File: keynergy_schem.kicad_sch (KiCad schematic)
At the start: 39 parts, among them J1 Conn_01x03_Pin, J2 Conn_01x03_Pin, J3 Conn_01x04_Pin, J4 Conn_01x03_Pin, J5 Conn_01x02_Pin, J6 Conn_01x03_Pin, J7 Conn_01x02_Pin, J8 Conn_01x03_Pin

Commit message: new
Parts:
- removed D1, D10, D11, D2, D3, D4, D5, D6, D7, D8, D9: D, Diode_THT:D_DO-35_SOD27_P7.62mm_Horizontal, symbol Device:D
- removed J2, J4, J6, J8: Conn_01x03_Pin, Connector_PinHeader_2.54mm:PinHeader_1x03_P2.54mm_Vertical, symbol Connector:Conn_01x03_Pin
- removed J5, J7: Conn_01x02_Pin, Connector_PinHeader_2.54mm:PinHeader_1x02_P2.54mm_Vertical, symbol Connector:Conn_01x02_Pin
- added C2: C_Polarized_Small, Capacitor_THT:CP_Radial_D8.0mm_P3.50mm, symbol Device:C_Polarized_Small
- added D1, D2, D3, D4: 1N5818, Diode_THT:D_DO-41_SOD81_P10.16mm_Horizontal, symbol Diode:1N5818
- added K12, K13, K14, K15, K16, K17, K18, K19, K20: ~, project library:Solenoid Key, symbol Key_symbol:Solenoid_Key
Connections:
- net Col 5-2 is gone; now on net Column 1: K9.4 (Bin)
- net Row 5-1 is gone; now on net Column 2: K10.4 (Bin)
- net Row 5-2 is gone; now on net Column 3: K11.4 (Bin)
- net Coil 2-1: now also K8.2 (C2); no longer K7.2 (C2)
- net Coil 5-1: now also K19.2 (C2); no longer K9.2 (C2)
- net Coil 5-2: now also K17.1 (C1); no longer K8.1 (C1)
- net Col 1-1: no longer K1.4 (Bin)
- net Col 1-2: no longer K2.4 (Bin)
- net Col 1-3: no longer K3.4 (Bin)
- net Col 1-4: no longer K4.4 (Bin)
- net Row 1: now also K1.3 (Bout), K2.3 (Bout), K3.3 (Bout), K4.3 (Bout)
- net Row 2: now also K5.3 (Bout), K6.3 (Bout), K7.3 (Bout), K8.3 (Bout)
- net Row 5: now also K17.3 (Bout), K18.3 (Bout), K19.3 (Bout), K20.3 (Bout)
- net Row 3: now reaches K11.3 (Bout)
- net Row 3: now also K10.3 (Bout), K9.3 (Bout), K12.3 (Bout)
- net Coil 3-2: now reaches K9.1 (C1)
- net Coil 3-2: no longer K8.2 (C2)
- net Coil 5-3 renamed Coil 3-1
- net Coil 5-4: no longer names the net of K10.1 (C1)
- net Coil 5-4: now also K9.2 (C2)
- net Col 2-1 renamed Column 1
- net Column 1: now also K1.4 (Bin), K13.4 (Bin), K17.4 (Bin)
- net Col 2-2 renamed Column 2
- net Column 2: now also K2.4 (Bin), K14.4 (Bin), K18.4 (Bin)
- net Col 2-3 renamed Column 3
- net Column 3: now also K3.4 (Bin), K15.4 (Bin), K19.4 (Bin)
- net Col 5-1 renamed Column 4
- net Column 4: now also K4.4 (Bin), K12.4 (Bin), K16.4 (Bin), K20.4 (Bin)
- new net: K17.2 (C2), K18.1 (C1)
- new net: K7.2 (C2), K8.1 (C1)
- new net: C2.2, D3.1 (K), D4.2 (A)
- new net: D1.2 (A), D3.2 (A)
- new net: K13.2 (C2), K14.1 (C1)
- new net: K14.2 (C2), K15.1 (C1)
- new net: C2.1, D2.1 (K), D4.1 (K)
- new net: D1.1 (K), D2.2 (A)
- new net: K18.2 (C2), K19.1 (C1)
- new net Coil 4-1: K15.2 (C2)
- new net Coil 4-2: K13.1 (C1)
- new net Row 4: K13.3 (Bout), K14.3 (Bout), K15.3 (Bout), K16.3 (Bout)
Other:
- note removed: "Row 1, Col 1-4"
- note removed: "Row 2-4, Col 1-3"
- note removed: "Row 2/3 - 4/5, Col 5"
- note removed: "Row 5, Col 1/2-3"
- moved on the sheet: A2, BT1, C1, D12, D13, D14, D15, J1, J3, K10, K11, K5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

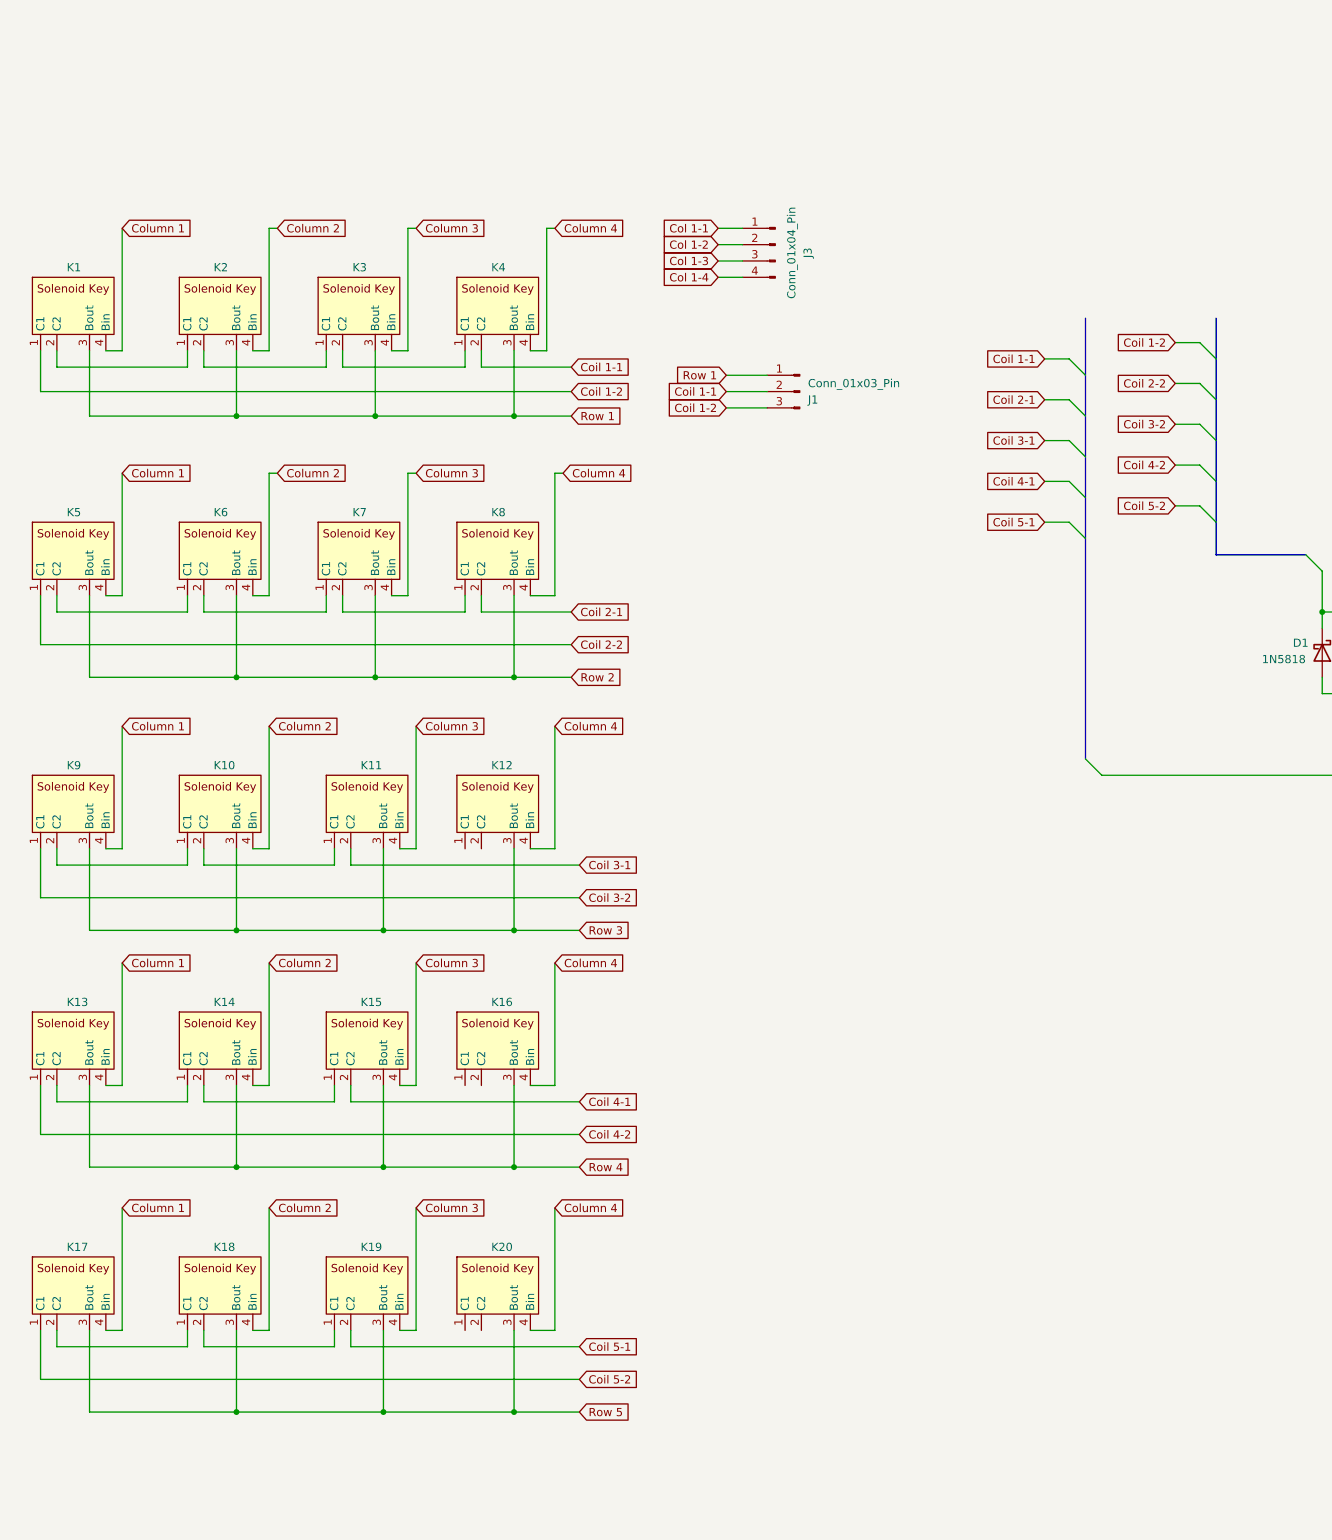
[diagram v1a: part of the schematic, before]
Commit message: new update
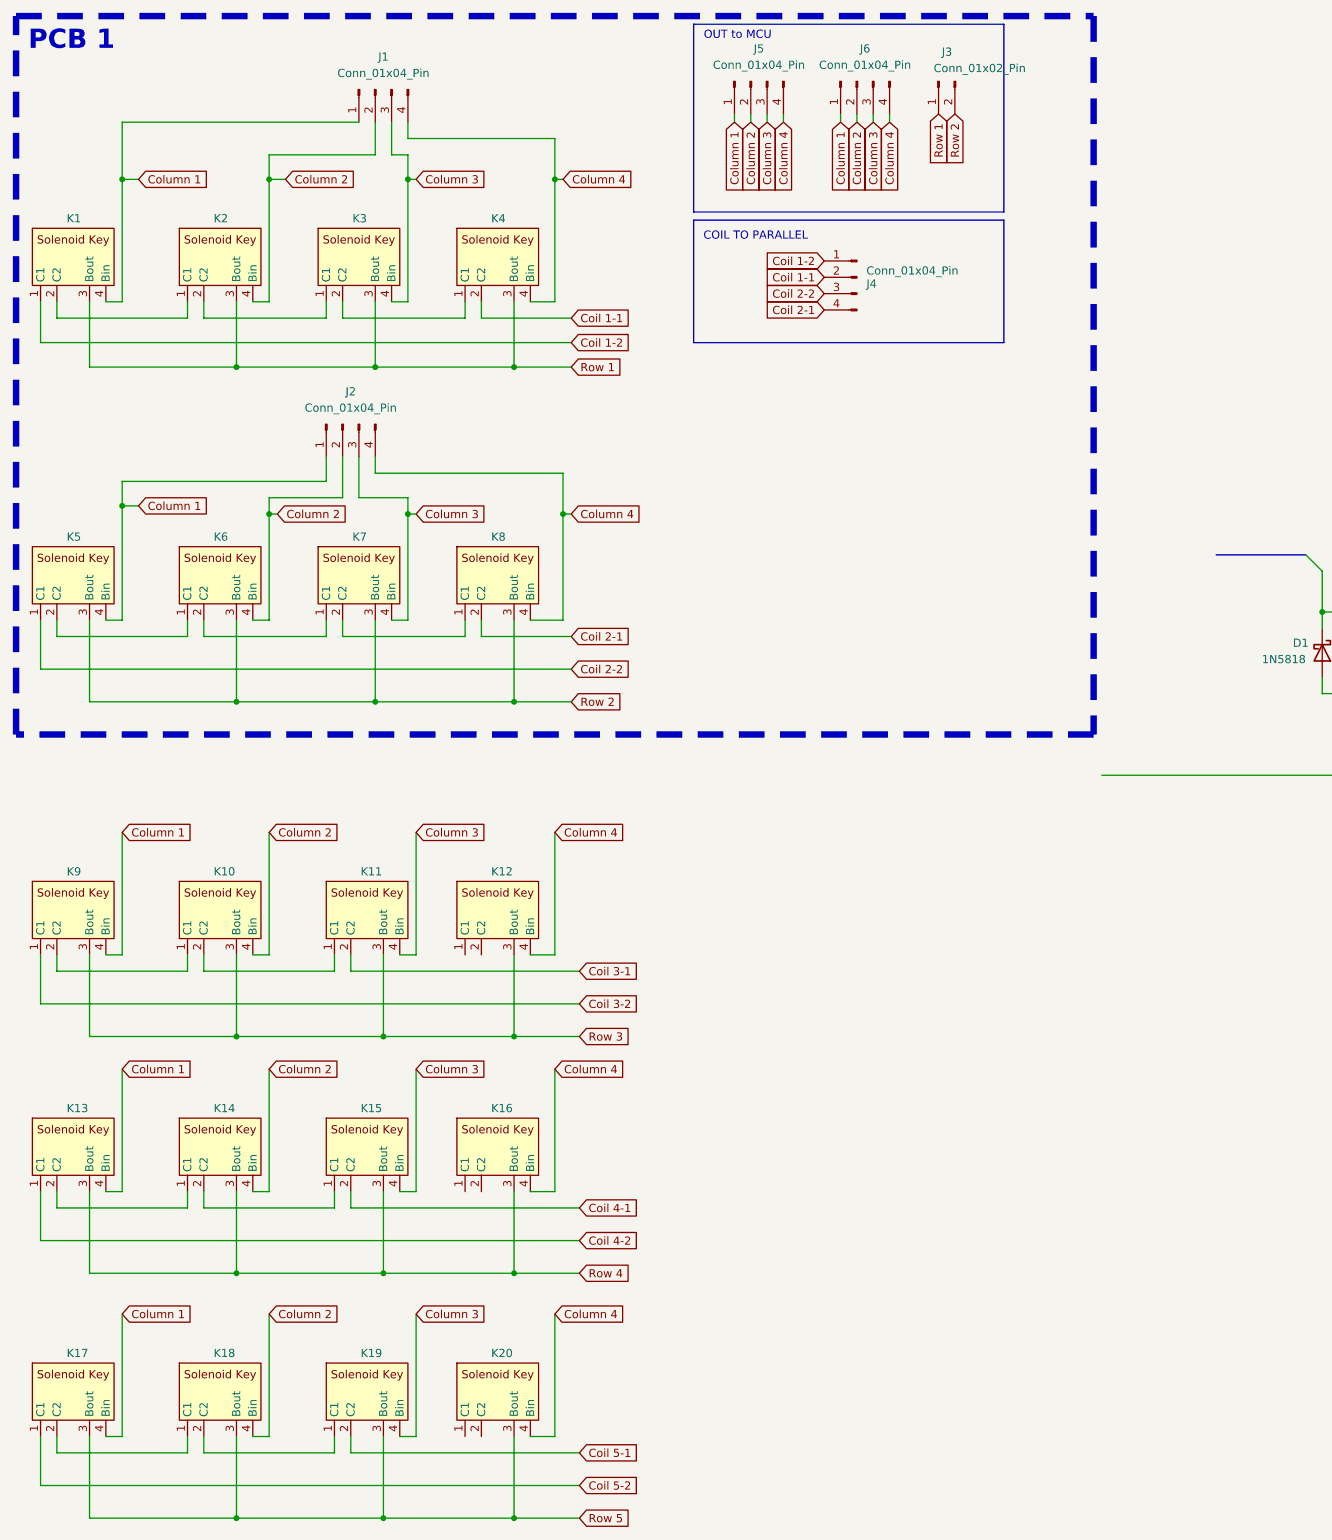
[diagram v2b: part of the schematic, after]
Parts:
- removed J1: Conn_01x03_Pin, Connector_PinHeader_2.54mm:PinHeader_1x03_P2.54mm_Vertical, symbol Connector:Conn_01x03_Pin
- added J2, J4, J5, J6: Conn_01x04_Pin, Connector_PinHeader_2.54mm:PinHeader_1x04_P2.54mm_Vertical, symbol Connector:Conn_01x04_Pin
- added J3: Conn_01x02_Pin, Connector_PinHeader_2.54mm:PinHeader_1x02_P2.54mm_Vertical, symbol Connector:Conn_01x02_Pin
- D1, D2, D3, D4: footprint Diode_THT:D_DO-41_SOD81_P10.16mm_Horizontal -> Diode_THT:D_DO-34_SOD68_P7.62mm_Horizontal
- renumbered J3 to J1
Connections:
- net Col 1-1 is gone; now on net Column 1: J1.1 (Pin_1)
- net Col 1-2 is gone; now on net Column 2: J1.2 (Pin_2)
- net Col 1-3 is gone; now on net Column 3: J1.3 (Pin_3)
- net Col 1-4 is gone; now on net Column 4: J1.4 (Pin_4)
- net Coil 1-1: now also J4.2 (Pin_2)
- net Coil 1-2: now also J4.1 (Pin_1)
- net Coil 2-1: now also J4.4 (Pin_4)
- net Coil 2-2: now also J4.3 (Pin_3)
- net Column 1: now also J2.1 (Pin_1), J5.1 (Pin_1), J6.1 (Pin_1)
- net Column 2: now also J2.2 (Pin_2), J5.2 (Pin_2), J6.2 (Pin_2)
- net Column 3: now also J2.3 (Pin_3), J5.3 (Pin_3), J6.3 (Pin_3)
- net Column 4: now also J2.4 (Pin_4), J5.4 (Pin_4), J6.4 (Pin_4)
- net Row 1: now also J3.1 (Pin_1)
- net Row 2: now also J3.2 (Pin_2)
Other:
- note added: "COIL TO PARALLEL"
- note added: "OUT to MCU"
- note added: "PCB 1"
- moved on the sheet: J1, K1, K10, K11, K12, K13, K14, K15, K16, K17, K18, K19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
